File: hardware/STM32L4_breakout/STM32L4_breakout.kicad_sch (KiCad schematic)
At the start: 67 parts, among them J1 12V IN, J10 GPIO, J12 USART1, J13 USART3, J14 UART4, J15 3.3V, J16 5V, J17 12V, J2 SWD, J3 Conn_01x08, J4 Conn_01x06, J5 Conn_01x10, J6 Conn_01x08, J7 I2C1, J8 I2C2, J9 I2C3, SW1 SW_SPDT, U1 LD1117S50TR_SOT223, U2 LD3985M33R_SOT23, U3 LD1117S33TR_SOT223, U4 STM32L476RGTx, X1 NX3215SA-32.768K

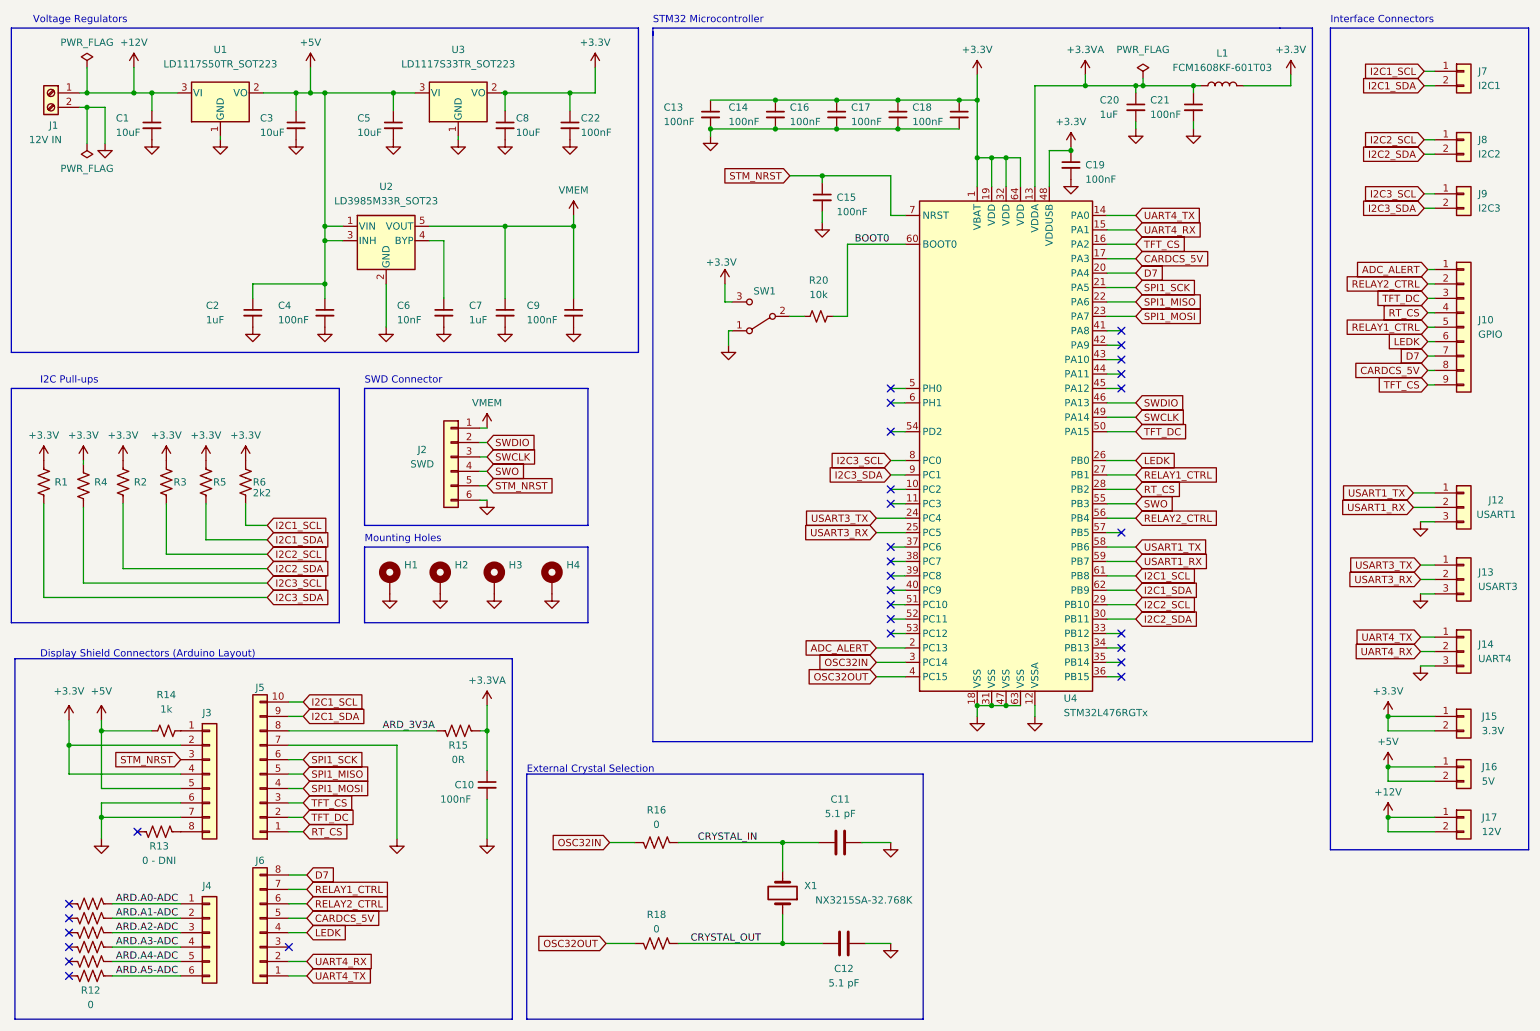
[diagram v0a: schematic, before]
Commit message: breakout board signal routing WIP
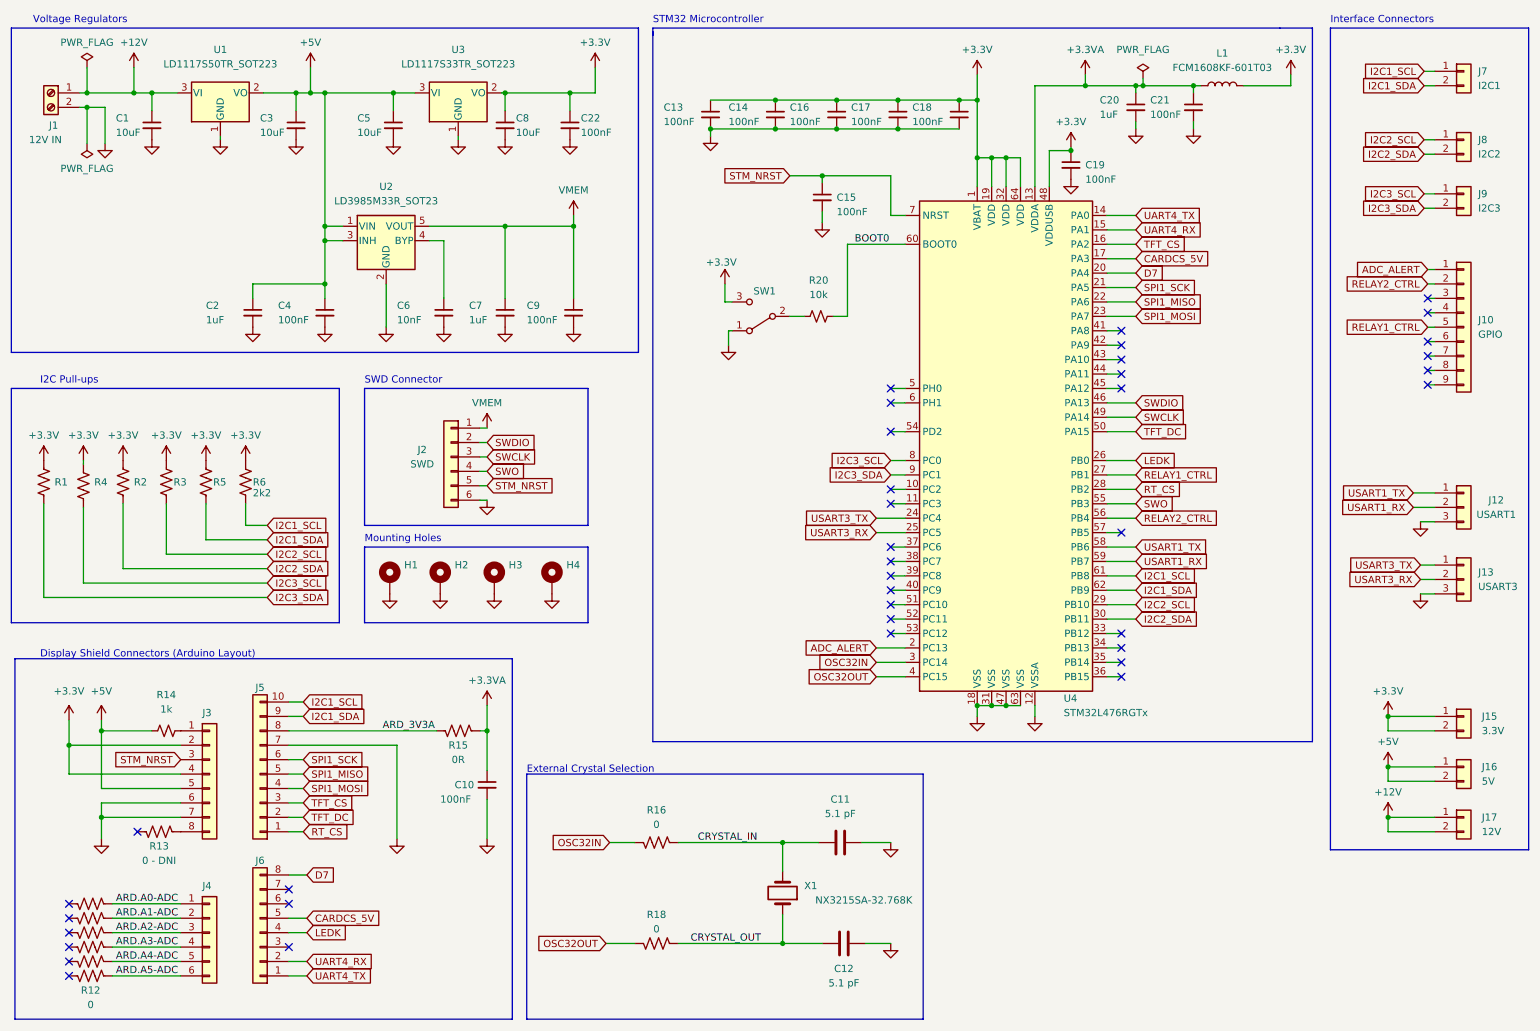
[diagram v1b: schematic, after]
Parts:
- removed J14: UART4, Connector_PinHeader_2.54mm:PinHeader_1x03_P2.54mm_Vertical, symbol Connector_Generic:Conn_01x03
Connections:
- net CARDCS_5V: no longer J10.8 (Pin_8)
- net D7: no longer J10.7 (Pin_7)
- net LEDK: no longer J10.6 (Pin_6)
- net RELAY1_CTRL: no longer J6.7 (Pin_7)
- net RELAY2_CTRL: no longer J6.6 (Pin_6)
- net RT_CS: no longer J10.4 (Pin_4)
- net TFT_CS: no longer J10.9 (Pin_9)
- net TFT_DC: no longer J10.3 (Pin_3)
- no-connect marks 30 -> 38
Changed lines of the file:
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@@
   (no_connect (at 168.91 82.55))
   (no_connect (at 168.91 90.17))
+  (no_connect (at 62.865 170.815))
   (no_connect (at 24.13 173.355))
   (no_connect (at 209.55 80.01))
   (no_connect (at 168.91 115.57))
   (no_connect (at 209.55 107.95))
+  (no_connect (at 263.525 69.215))
   (no_connect (at 209.55 128.27))
   (no_connect (at 168.91 113.03))
@@
   (no_connect (at 168.91 120.65))
   (no_connect (at 209.55 74.93))
+  (no_connect (at 263.525 81.915))
+  (no_connect (at 263.525 66.675))
+  (no_connect (at 263.525 79.375))
   (no_connect (at 209.55 130.81))
   (no_connect (at 168.91 123.19))
+  (no_connect (at 263.525 76.835))
   (no_connect (at 168.91 125.73))
   (no_connect (at 24.13 180.975))
+  (no_connect (at 263.525 74.295))
   (no_connect (at 209.55 82.55))
   (no_connect (at 36.195 160.655))
   (no_connect (at 168.91 85.09))
   (no_connect (at 168.91 102.87))
+  (no_connect (at 62.865 173.355))
   (no_connect (at 24.13 175.895))
   (no_connect (at 209.55 133.35))
@@
     (stroke (width 0) (type default) (color 0 0 0 0))
   )
-  (wire (pts (xy 262.255 126.365) (xy 264.795 126.365))
-    (stroke (width 0) (type default) (color 0 0 0 0))
-  )
   (wire (pts (xy 64.135 30.48) (xy 64.135 33.655))
     (stroke (width 0) (type default) (color 0 0 0 0))
@@
     (stroke (width 0) (type default) (color 0 0 0 0))
   )
-  (wire (pts (xy 262.255 131.445) (xy 264.795 131.445))
-    (stroke (width 0) (type default) (color 0 0 0 0))
-  )
   (wire (pts (xy 262.89 41.275) (xy 264.795 41.275))
     (stroke (width 0) (type default) (color 0 0 0 0))
@@
     (stroke (width 0) (type default) (color 0 0 0 0))
   )
-  (wire (pts (xy 62.865 173.355) (xy 66.04 173.355))
-    (stroke (width 0) (type default) (color 0 0 0 0))
-  )
   (wire (pts (xy 50.8 38.1) (xy 50.8 38.735))
     (stroke (width 0) (type default) (color 0 0 0 0))
@@
     (stroke (width 0) (type default) (color 0 0 0 0))
   )
-  (wire (pts (xy 262.255 128.905) (xy 264.795 128.905))
-    (stroke (width 0) (type default) (color 0 0 0 0))
-  )
   (wire (pts (xy 118.745 180.34) (xy 123.825 180.34))
     (stroke (width 0) (type default) (color 0 0 0 0))
@@
     (stroke (width 0) (type default) (color 0 0 0 0))
   )
-  (wire (pts (xy 62.865 170.815) (xy 66.04 170.815))
-    (stroke (width 0) (type default) (color 0 0 0 0))
-  )
   (wire (pts (xy 65.405 150.495) (xy 62.865 150.495))
     (stroke (width 0) (type default) (color 0 0 0 0))
@@
     (effects (font (size 1.27 1.27)) (justify left bottom))
   )
-  (global_label "CARDCS_5V" (shape input) (at 263.525 79.375 180) (fields_autoplaced)
-    (effects (font (size 1.27 1.27)) (justify right))
-    (property "Intersheet References" "${INTERSHEET_REFS}" (id 0) (at 250.4681 79.4544 0)
-      (effects (font (size 1.27 1.27)) (justify right) hide)
-    )
-  )
   (global_label "RELAY1_CTRL" (shape input) (at 263.525 71.755 180) (fields_autoplaced)
     (effects (font (size 1.27 1.27)) (justify right))
@@
     )
   )
-  (global_label "TFT_CS" (shape input) (at 263.525 81.915 180) (fields_autoplaced)
-    (effects (font (size 1.27 1.27)) (justify right))
-    (property "Intersheet References" "${INTERSHEET_REFS}" (id 0) (at 254.6409 81.8356 0)
-      (effects (font (size 1.27 1.27)) (justify right) hide)
-    )
-  )
   (global_label "STM_NRST" (shape input) (at 97.79 99.695 0) (fields_autoplaced)
     (effects (font (size 1.27 1.27)) (justify left))
@@
     )
   )
-  (global_label "RT_CS" (shape input) (at 263.525 69.215 180) (fields_autoplaced)
-    (effects (font (size 1.27 1.27)) (justify right))
-    (property "Intersheet References" "${INTERSHEET_REFS}" (id 0) (at 255.4271 69.1356 0)
-      (effects (font (size 1.27 1.27)) (justify right) hide)
-    )
-  )
   (global_label "CARDCS_5V" (shape input) (at 66.04 175.895 0) (fields_autoplaced)
     (effects (font (size 1.27 1.27)) (justify left))
@@
     )
   )
-  (global_label "D7" (shape input) (at 263.525 76.835 180) (fields_autoplaced)
-    (effects (font (size 1.27 1.27)) (justify right))
-    (property "Intersheet References" "${INTERSHEET_REFS}" (id 0) (at 258.6324 76.7556 0)
-      (effects (font (size 1.27 1.27)) (justify right) hide)
-    )
-  )
   (global_label "RT_CS" (shape input) (at 65.405 160.655 0) (fields_autoplaced)
     (effects (font (size 1.27 1.27)) (justify left))
@@
     )
   )
-  (global_label "RELAY2_CTRL" (shape input) (at 66.04 173.355 0) (fields_autoplaced)
-    (effects (font (size 1.27 1.27)) (justify left))
-    (property "Intersheet References" "${INTERSHEET_REFS}" (id 0) (at 80.7902 173.2756 0)
-      (effects (font (size 1.27 1.27)) (justify left) hide)
-    )
-  )
   (global_label "I2C3_SCL" (shape input) (at 262.89 48.26 180) (fields_autoplaced)
     (effects (font (size 1.27 1.27)) (justify right))
@@
     )
   )
-  (global_label "UART4_TX" (shape input) (at 262.255 126.365 180) (fields_autoplaced)
-    (effects (font (size 1.27 1.27)) (justify right))
-    (property "Intersheet References" "${INTERSHEET_REFS}" (id 0) (at 250.8309 126.2856 0)
-      (effects (font (size 1.27 1.27)) (justify right) hide)
-    )
-  )
   (global_label "SPI1_MOSI" (shape input) (at 65.405 153.035 0) (fields_autoplaced)
     (effects (font (size 1.27 1.27)) (justify left))
@@
     )
   )
-  (global_label "RELAY1_CTRL" (shape input) (at 66.04 170.815 0) (fields_autoplaced)
-    (effects (font (size 1.27 1.27)) (justify left))
-    (property "Intersheet References" "${INTERSHEET_REFS}" (id 0) (at 80.7902 170.7356 0)
-      (effects (font (size 1.27 1.27)) (justify left) hide)
-    )
-  )
   (global_label "USART1_RX" (shape input) (at 212.09 113.03 0) (fields_autoplaced)
     (effects (font (size 1.27 1.27)) (justify left))
@@
     )
   )
-  (global_label "UART4_RX" (shape input) (at 262.255 128.905 180) (fields_autoplaced)
-    (effects (font (size 1.27 1.27)) (justify right))
-    (property "Intersheet References" "${INTERSHEET_REFS}" (id 0) (at 250.5286 128.8256 0)
-      (effects (font (size 1.27 1.27)) (justify right) hide)
-    )
-  )
   (global_label "SPI1_SCK" (shape input) (at 212.09 64.77 0) (fields_autoplaced)
     (effects (font (size 1.27 1.27)) (justify left))
@@
     )
   )
-  (global_label "TFT_DC" (shape input) (at 263.525 66.675 180) (fields_autoplaced)
-    (effects (font (size 1.27 1.27)) (justify right))
-    (property "Intersheet References" "${INTERSHEET_REFS}" (id 0) (at 254.5805 66.5956 0)
-      (effects (font (size 1.27 1.27)) (justify right) hide)
-    )
-  )
   (global_label "OSC32IN" (shape input) (at 166.37 130.81 180) (fields_autoplaced)
     (effects (font (size 1.27 1.27)) (justify right))
@@
     )
   )
-  (global_label "LEDK" (shape input) (at 263.525 74.295 180) (fields_autoplaced)
-    (effects (font (size 1.27 1.27)) (justify right))
-    (property "Intersheet References" "${INTERSHEET_REFS}" (id 0) (at 256.3948 74.2156 0)
-      (effects (font (size 1.27 1.27)) (justify right) hide)
-    )
-  )
   (global_label "I2C1_SDA" (shape input) (at 59.055 109.22 0) (fields_autoplaced)
     (effects (font (size 1.27 1.27)) (justify left))
@@
     (pin "2")
   )
-  (symbol (lib_id "power:GND") (at 262.255 131.445 0) (unit 1)
-    (in_bom yes) (on_board yes) (fields_autoplaced)
-    (property "Reference" "#PWR043" (id 0) (at 262.255 137.795 0)
-      (effects (font (size 1.27 1.27)) hide)
-    )
-    (property "Value" "GND" (id 1) (at 262.255 136.525 0)
-      (effects (font (size 1.27 1.27)) hide)
-    )
-    (property "Footprint" "" (id 2) (at 262.255 131.445 0)
-      (effects (font (size 1.27 1.27)) hide)
-    )
-    (property "Datasheet" "" (id 3) (at 262.255 131.445 0)
-      (effects (font (size 1.27 1.27)) hide)
-    )
-    (pin "1")
-  )
   (symbol (lib_id "power:PWR_FLAG") (at 213.36 27.94 0) (unit 1)
     (in_bom yes) (on_board yes) (fields_autoplaced)
@@
     (pin "1")
   )
-  (symbol (lib_id "Connector_Generic:Conn_01x03") (at 269.875 128.905 0) (unit 1)
-    (in_bom yes) (on_board yes)
-    (property "Reference" "J14" (id 0) (at 272.415 127.6349 0)
-      (effects (font (size 1.27 1.27)) (justify left))
-    )
-    (property "Value" "UART4" (id 1) (at 272.415 130.1749 0)
-      (effects (font (size 1.27 1.27)) (justify left))
-    )
-    (property "Footprint" "Connector_PinHeader_2.54mm:PinHeader_1x03_P2.54mm_Vertical" (id 2) (at 269.875 128.905 0)
-      (effects (font (size 1.27 1.27)) hide)
-    )
-    (property "Datasheet" "~" (id 3) (at 269.875 128.905 0)
-      (effects (font (size 1.27 1.27)) hide)
-    )
-    (pin "1")
-    (pin "2")
-    (pin "3")
-  )
   (symbol (lib_id "power:+3.3V") (at 55.245 95.25 0) (unit 1)
     (in_bom yes) (on_board yes)
@@
       (reference "#PWR042") (unit 1) (value "GND") (footprint "")
     )
-    (path "/4a8094da-141b-4e22-9942-80faa75cb312"
-      (reference "#PWR043") (unit 1) (value "GND") (footprint "")
-    )
     (path "/5faa3663-1cde-4241-a4ce-4f79e7fbfe0a"
       (reference "#PWR044") (unit 1) (value "GND") (footprint "")
@@
       (reference "J13") (unit 1) (value "USART3") (footprint "Connector_PinHeader_2.54mm:PinHeader_1x03_P2.54mm_Vertical")
     )
-    (path "/70b380d3-3856-4255-af62-fd9df70ff722"
-      (reference "J14") (unit 1) (value "UART4") (footprint "Connector_PinHeader_2.54mm:PinHeader_1x03_P2.54mm_Vertical")
-    )
     (path "/ea8310bc-b60d-4fa4-a884-85caa2804f75"
